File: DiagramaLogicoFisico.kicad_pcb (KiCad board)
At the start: 2 copper layers, 87.6 x 95.2 mm, 40 parts, among them J1 Conn_01x02_Servo1, J2 Conn_01x03_UART1, J3 Conn_01x03_UART2, J4 Conn_01x04_PWM, J5 Conn_01x05_PROGRAMER, J6 Conn_01x02_POWER, J7 Conn_01x02_Servo2, J8 Conn_01x02_Servo3, J9 Conn_01x02_Servo4, U2 DSPIC33EP128GM604, U3 LM317T/SERVO, U4 LM317T/SERVO, U5 LM317T/SERVO, U6 LM317T/SERVO, U7 LM317T/DSPIC, Y1 7.3728Mhz

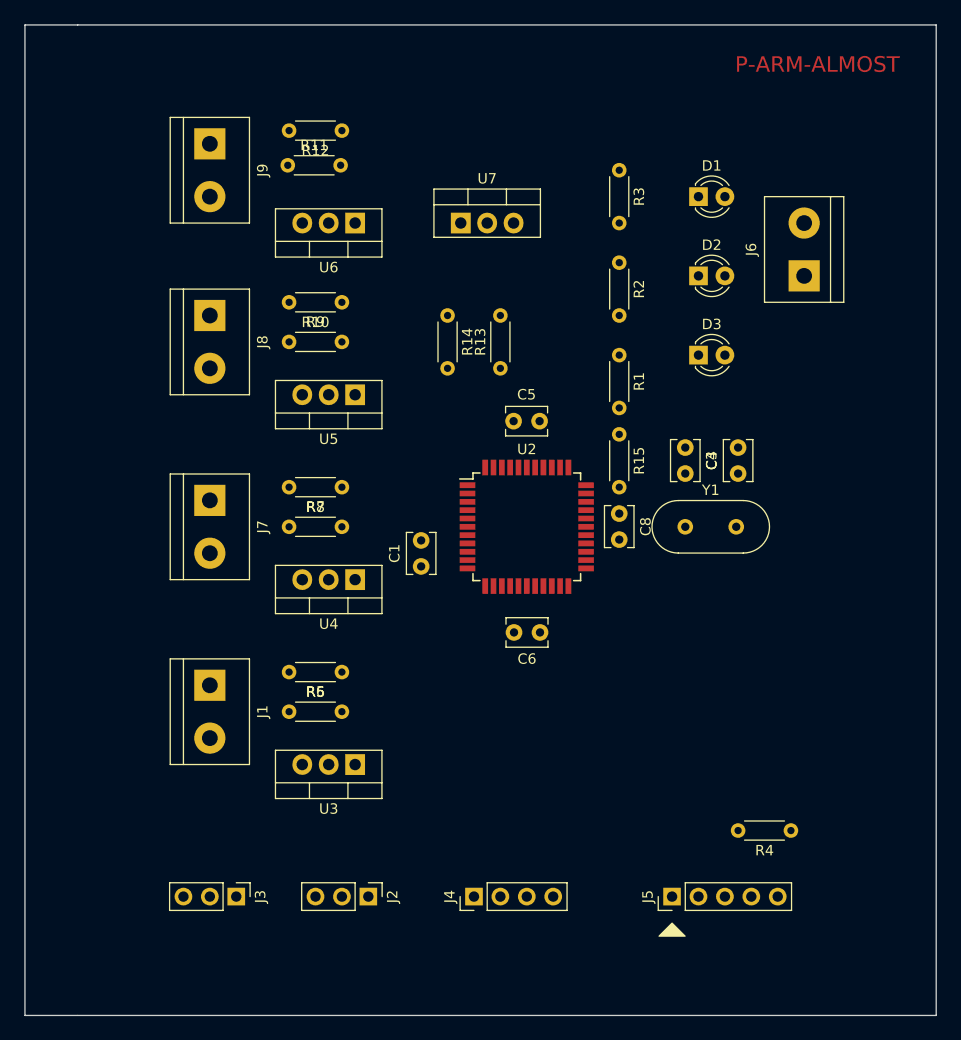
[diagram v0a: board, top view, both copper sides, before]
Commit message: Proyecto Almost Released Vias
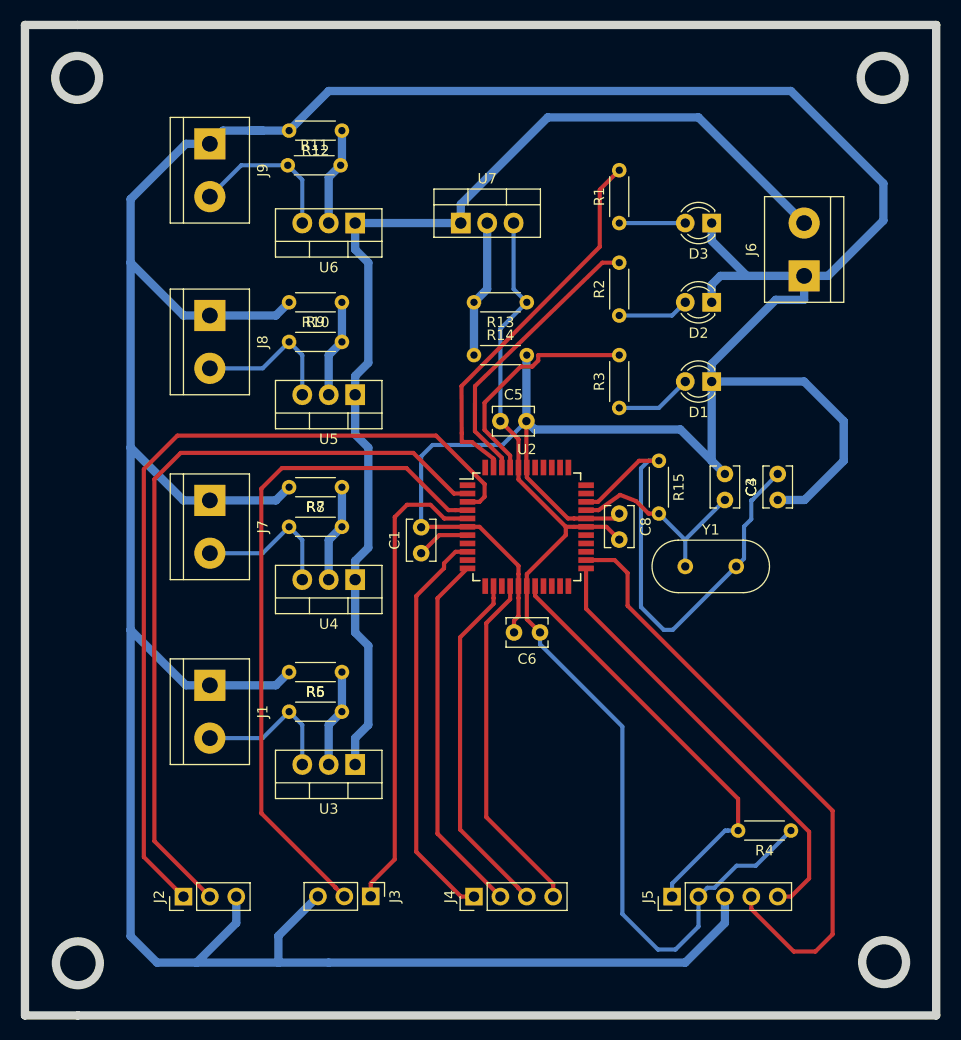
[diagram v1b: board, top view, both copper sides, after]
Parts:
- added G***: LOGO, Logo:logoUni, F.Cu at (158.8, 62.0)
- added G***: LOGO, Logo:logo2, F.Cu at (202.4, 66.0)
- moved R3 22.9 mm to (191.8, 95.2), turned to 90 degrees
- moved D1 17.8 mm to (200.7, 92.7), turned to 180 degrees
- moved J2 17.8 mm to (149.9, 142.2), turned to 90 degrees
- moved J3 12.9 mm to (167.9, 142.2)
- moved D3 12.8 mm to (200.7, 77.5), turned to 180 degrees
- moved R1 12.7 mm to (191.8, 77.5), turned to 90 degrees
- moved R13 6.84 mm to (182.9, 85.1), turned to 180 degrees
- moved R2 5.08 mm to (191.8, 86.4), turned to 90 degrees
- moved R14 4.58 mm to (177.8, 90.2), turned to 0 degrees
- moved C3 4.58 mm to (207.0, 104.1)
- moved C4 4.58 mm to (201.9, 101.6)
- moved R15 4.58 mm to (195.6, 100.3)
- moved Y1 3.81 mm to (198.1, 110.5)
- moved D2 2.84 mm to (200.7, 85.1), turned to 180 degrees
- moved C5 1.27 mm to (180.3, 96.5)
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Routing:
- net GND: track 0.00 -> 443.9 mm
- net Net-(J6-Pad2): track 0.00 -> 107.9 mm
- net +3V3: track 0.00 -> 105.7 mm
- net Net-(J2-Pad1): track 0.00 -> 81.8 mm
- net Net-(J2-Pad2): track 0.00 -> 75.1 mm
- net Net-(J3-Pad2): track 0.00 -> 64.8 mm
- net Net-(J5-Pad4): track 0.00 -> 58.8 mm
- net Net-(C3-Pad2): track 0.00 -> 47.1 mm
- net Net-(J3-Pad1): track 0.00 -> 45.5 mm
- net Net-(J5-Pad5): track 0.00 -> 42.4 mm
- net Net-(J5-Pad1): track 0.00 -> 41.3 mm
- net Net-(J4-Pad1): track 0.00 -> 38.9 mm
- net Net-(R1-Pad2): track 0.00 -> 36.8 mm
- net Net-(J4-Pad2): track 0.00 -> 35.3 mm
- net Net-(J4-Pad3): track 0.00 -> 33.9 mm
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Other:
- outline, holes or cut-outs redrawn
- board text added: "DSPIC"
- board text added: "P-ARM ALMOST"
- board text added: "POWER"
- board text added: "PROBE"
- board text added: "PWM"
- board text added: "SERVO 1"
- board text added: "SERVO 2"
- board text added: "SERVO 3"
- board text added: "SERVO 4"
- board text added: "TM"
- board text added: "UART1"
- board text added: "UART2"
- board text added: "by NPCMOS"
- board text added: "Δ"
- board text removed: "P-ARM-ALMOST"
